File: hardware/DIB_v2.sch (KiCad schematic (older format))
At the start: 1 part, among them J6 Conn_02x10_Odd_Even

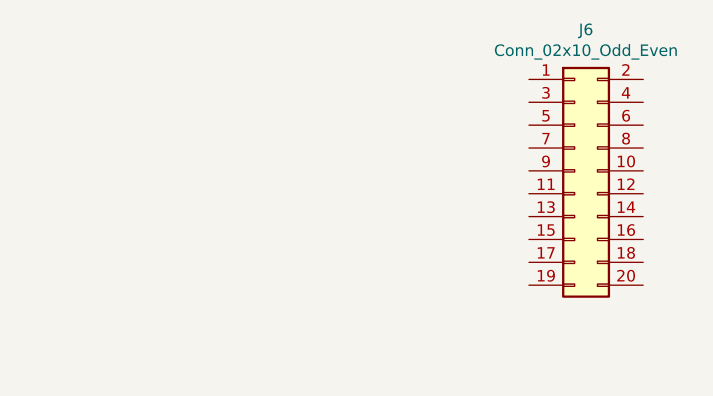
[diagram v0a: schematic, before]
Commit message: Adding last known changes to shematics
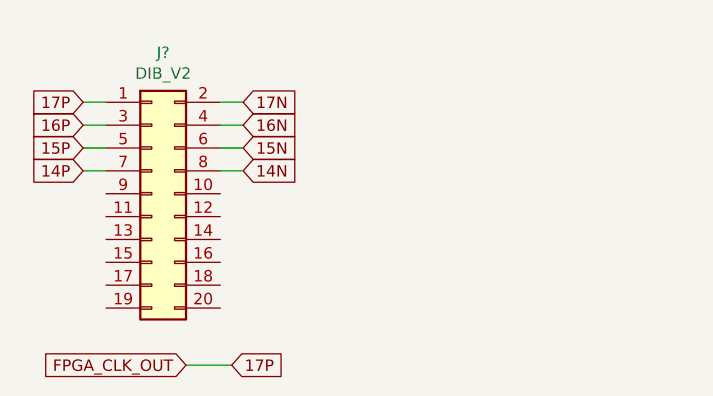
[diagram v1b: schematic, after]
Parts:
- removed J6: Conn_02x10_Odd_Even, Connector_PinHeader_2.54mm:PinHeader_2x10_P2.54mm_Horizontal, symbol Connector_Generic:Conn_02x10_Odd_Even
- added J?: DIB_V2, Connector_PinHeader_2.54mm:PinHeader_2x10_P2.54mm_Horizontal, symbol Connector_Generic:Conn_02x10_Odd_Even
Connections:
- new net 14N: J?.8 (Pin_8)
- new net 14P: J?.7 (Pin_7)
- new net 15N: J?.6 (Pin_6)
- new net 15P: J?.5 (Pin_5)
- new net 16N: J?.4 (Pin_4)
- new net 16P: J?.3 (Pin_3)
- new net 17N: J?.2 (Pin_2)
- new net 17P: J?.1 (Pin_1)
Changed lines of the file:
@@
 $Descr A4 11693 8268
 encoding utf-8
-Sheet 5 11
+Sheet 5 10
 Title ""
-Date ""
-Rev ""
-Comp ""
+Date "2020-01-29"
+Rev "0.1"
+Comp "Envox d.o.o."
 Comment1 ""
 Comment2 ""
@@
 Comment4 ""
 $EndDescr
+Text GLabel 1950 2350 0    50   Input ~ 0
+FPGA_CLK_OUT
+Text GLabel 2150 2350 2    50   Input ~ 0
+17P
+Wire Wire Line
+	2150 2350 1950 2350
 $Comp
-L Connector_Generic:Conn_02x10_Odd_Even J6
-U 1 1 5E2F30CC
-P 3650 1500
-F 0 "J6" H 3700 2117 50  0000 C CNN
-F 1 "Conn_02x10_Odd_Even" H 3700 2026 50  0000 C CNN
-F 2 "Connector_PinHeader_2.54mm:PinHeader_2x10_P2.54mm_Horizontal" H 3650 1500 50  0001 C CNN
-F 3 "~" H 3650 1500 50  0001 C CNN
-	1    3650 1500
+L Connector_Generic:Conn_02x10_Odd_Even J?
+U 1 1 5E84CF5B
+P 1800 1600
+AR Path="/5E22D00E/5E84CF5B" Ref="J?"  Part="1"
+AR Path="/5E22C01C/5E84CF5B" Ref="J?"  Part="1"
+F 0 "J?" H 1850 2217 50  0000 C CNN
+F 1 "DIB_V2" H 1850 2126 50  0000 C CNN
+F 2 "Connector_PinHeader_2.54mm:PinHeader_2x10_P2.54mm_Horizontal" H 1800 1600 50  0001 C CNN
+F 3 "~" H 1800 1600 50  0001 C CNN
+	1    1800 1600
 	1    0    0    -1
 $EndComp
+Text GLabel 1500 1200 0    50   Input ~ 0
+17P
+Text GLabel 1500 1300 0    50   Input ~ 0
+16P
+Text GLabel 1500 1400 0    50   Input ~ 0
+15P
+Text GLabel 1500 1500 0    50   Input ~ 0
+14P
+Text GLabel 2200 1200 2    50   Input ~ 0
+17N
+Text GLabel 2200 1300 2    50   Input ~ 0
+16N
+Text GLabel 2200 1400 2    50   Input ~ 0
+15N
+Text GLabel 2200 1500 2    50   Input ~ 0
+14N
+Wire Wire Line
+	1500 1200 1600 1200
+Wire Wire Line
+	1500 1300 1600 1300
+Wire Wire Line
+	1500 1400 1600 1400
+Wire Wire Line
+	1500 1500 1600 1500
+Wire Wire Line
+	2100 1200 2200 1200
+Wire Wire Line
+	2100 1300 2200 1300
+Wire Wire Line
+	2100 1400 2200 1400
+Wire Wire Line
+	2100 1500 2200 1500
 $EndSCHEMATC
